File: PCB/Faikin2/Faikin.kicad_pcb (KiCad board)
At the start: 2 copper layers, 70 x 70 mm, 30 parts, among them J1 1x5, J3 Shelly, Q1 BSS138PS, U2 Barcode, U3 MD8942, U4 ESP32-S3-MINI-1

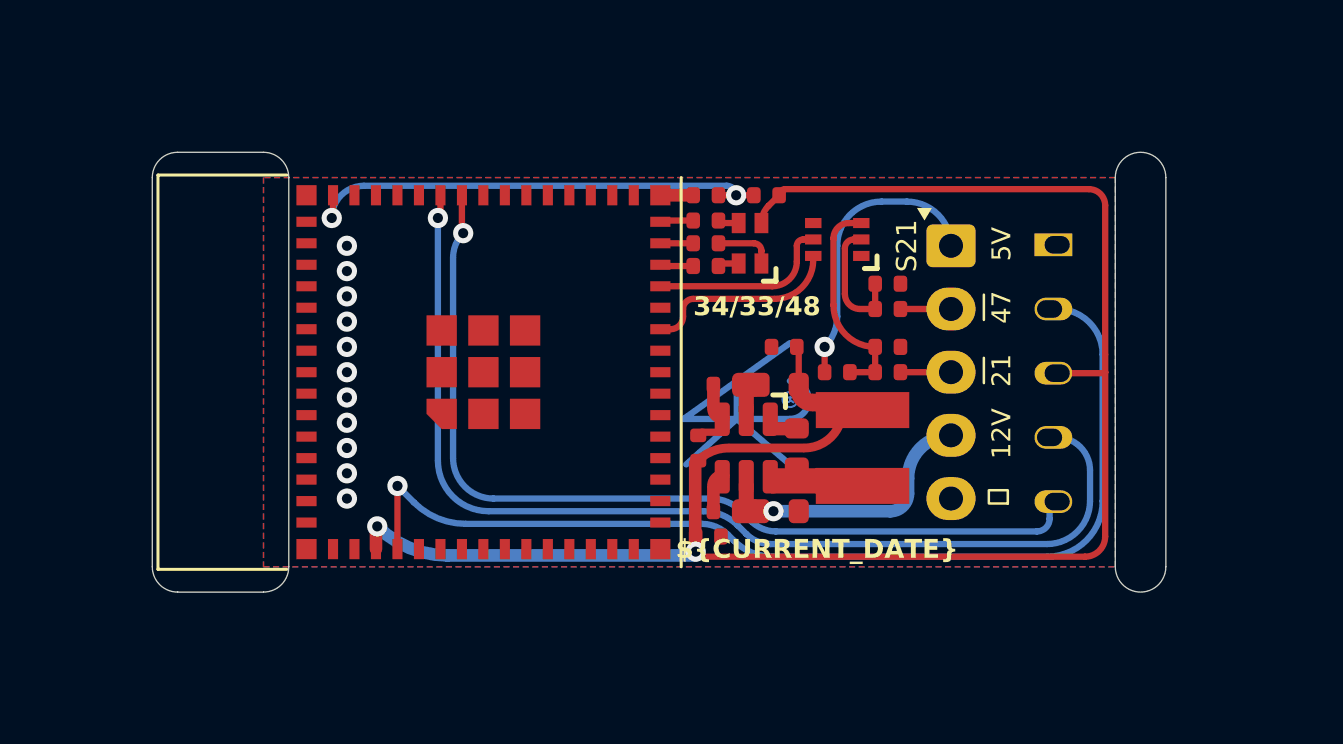
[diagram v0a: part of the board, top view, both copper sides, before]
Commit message: SMaller
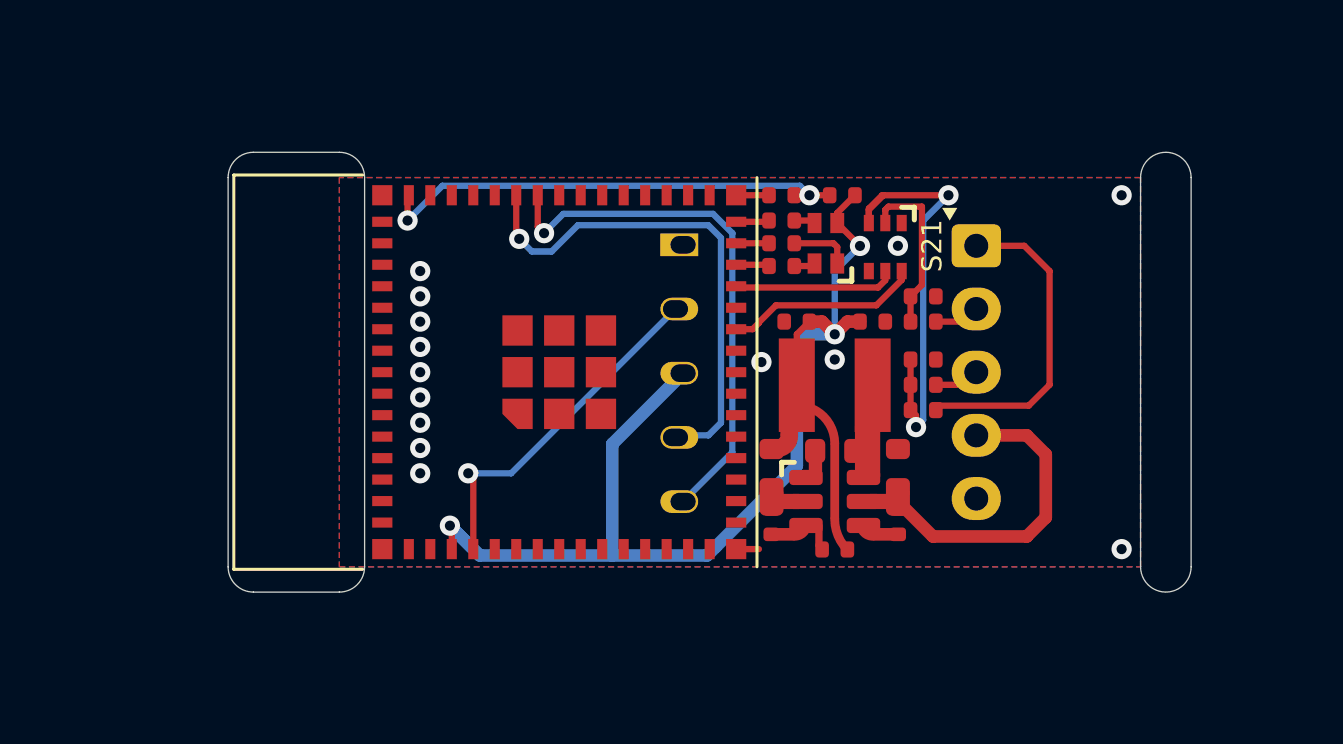
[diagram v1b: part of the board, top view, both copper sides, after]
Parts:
- removed Logo1: AJK, RevK:AJK
- moved J3 14.8 mm to (133.8, 61.0)
- moved C2 9.19 mm to (138.5, 59.0), turned to 180 degrees
- moved R11 6.81 mm to (142.5, 66.9), turned to -90 degrees
- moved R9 6.73 mm to (140.0, 68.0), turned to 0 degrees
- moved R10 5.71 mm to (137.5, 66.9), turned to -90 degrees
- moved C8 4.99 mm to (142.5, 64.8), turned to 90 degrees
- moved U3 4.09 mm to (140.0, 66.1), turned to 180 degrees
- moved R1 3.72 mm to (143.5, 62.5), turned to 180 degrees
- moved C5 3.64 mm to (141.5, 59.0), turned to 0 degrees
- moved C9 3.33 mm to (137.5, 64.8), turned to -90 degrees
- moved C6 3.00 mm to (137.9, 54.0)
- moved D2 3.00 mm to (139.7, 55.9)
- moved R12 3.00 mm to (137.9, 55.0)
- moved R3 3.00 mm to (140.3, 54.0)
- moved R5 3.00 mm to (137.9, 55.9)
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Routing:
- net Net-(J3-0): track 41.0 -> 14.0 mm
- net Net-(J3-Rx): track 41.9 -> 19.8 mm
- net +3.3V: track 65.9 -> 44.3 mm, vias 2 -> 3
- net Net-(J3-Tx): track 36.3 -> 21.1 mm
- net Net-(Q1B-SP): track 8.59 -> 17.7 mm, vias 0 -> 2
- net DC: track 9.45 -> 12.3 mm, vias 1 -> 0
- net Net-(Q1A-GN): track 5.15 -> 6.76 mm
- net Net-(J1-Pin_1): track 11.5 -> 12.7 mm, vias 1 -> 0
- net GND: track 1.20 -> 2.20 mm, vias 11 -> 14
- net TX: track 7.33 -> 6.33 mm
- net Net-(J1-Pin_3): track 2.00 -> 1.10 mm
- net Net-(J1-Pin_2): track 2.00 -> 1.10 mm
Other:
- board text added: "A"
- board text added: "RGB: 34/33/48"
- board text removed: "21"
- board text removed: "34/33/48"
- board text removed: "47"
